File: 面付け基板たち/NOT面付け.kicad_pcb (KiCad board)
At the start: 2 copper layers, 62.9 x 53.3 mm, 45 parts, among them J1 Conn_01x01, J2 Conn_01x02, J3 Conn_01x02

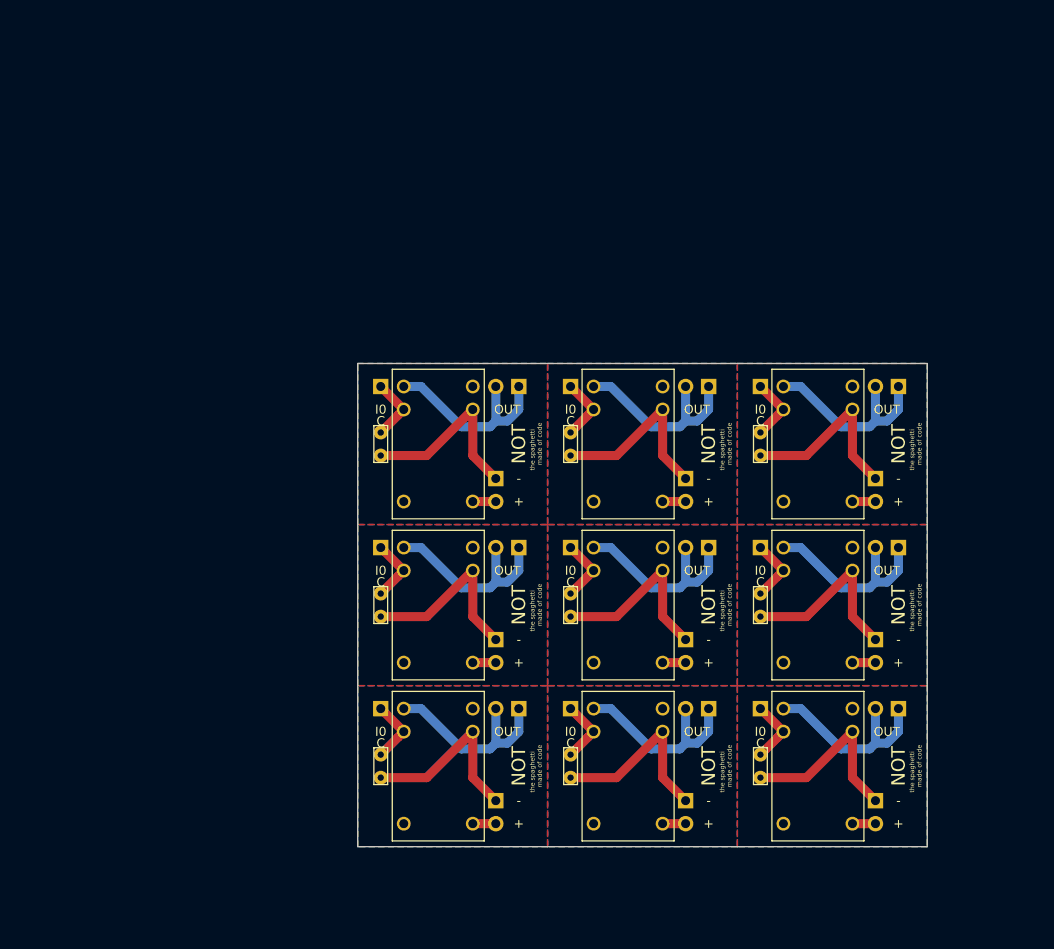
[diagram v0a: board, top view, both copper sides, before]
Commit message: Add files via upload
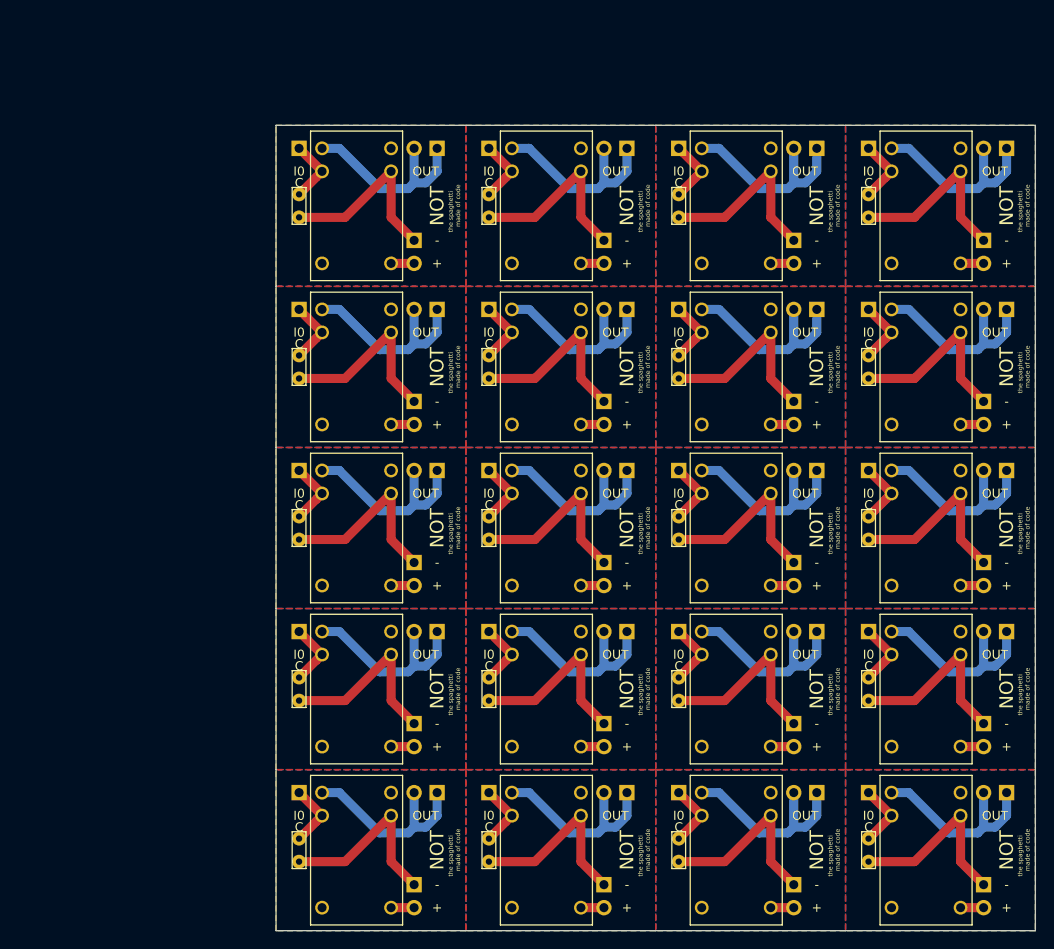
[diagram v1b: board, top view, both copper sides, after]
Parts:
- removed the C1 at (117.5, 116.2)
- removed the C1 at (96.5, 116.2)
- removed the C1 at (75.6, 116.2)
- removed the C1 at (117.5, 98.4)
- removed the C1 at (96.5, 98.4)
- removed the C1 at (75.6, 98.4)
- removed the C1 at (117.5, 80.6)
- removed the C1 at (96.5, 80.6)
- removed the J1 at (117.5, 108.6)
- removed the J1 at (96.5, 108.6)
- removed the J1 at (75.6, 108.6)
- removed the J1 at (117.5, 90.8)
- removed the J1 at (96.5, 90.8)
- removed the J1 at (75.6, 90.8)
- removed the J1 at (117.5, 73.0)
- removed the J1 at (96.5, 73.0)
- removed the J2 at (132.7, 108.6)
- removed the J2 at (111.8, 108.6)
- removed the J2 at (90.8, 108.6)
- removed the J2 at (132.7, 90.8)
- removed the J2 at (111.8, 90.8)
- removed the J2 at (90.8, 90.8)
- removed the J2 at (132.7, 73.0)
- removed the J2 at (111.8, 73.0)
- removed the J3 at (130.2, 118.7)
- removed the J3 at (109.2, 118.7)
- removed the J3 at (88.3, 118.7)
- removed the J3 at (130.2, 101.0)
- removed the J3 at (109.2, 101.0)
- removed the J3 at (88.3, 101.0)
- removed the J3 at (130.2, 83.2)
- removed the J3 at (109.2, 83.2)
- removed the SPDT1 at (125.1, 113.7)
- removed the SPDT1 at (104.1, 113.7)
- removed the SPDT1 at (83.2, 113.7)
- removed the SPDT1 at (125.1, 95.9)
- removed the SPDT1 at (104.1, 95.9)
- removed the SPDT1 at (83.2, 95.9)
- removed the SPDT1 at (125.1, 78.1)
- removed the SPDT1 at (104.1, 78.1)
- added C1: C, MiyakeFootprintLib:Condensor, F.Cu at (129.4, 125.5)
- added C1: C, MiyakeFootprintLib:Condensor, F.Cu at (108.5, 89.9)
- added C1: C, MiyakeFootprintLib:Condensor, F.Cu at (87.5, 89.9)
- added C1: C, MiyakeFootprintLib:Condensor, F.Cu at (66.5, 89.9)
- added C1: C, MiyakeFootprintLib:Condensor, F.Cu at (129.4, 72.1)
- added C1: C, MiyakeFootprintLib:Condensor, F.Cu at (108.5, 72.1)
- added C1: C, MiyakeFootprintLib:Condensor, F.Cu at (87.5, 72.1)
- added C1: C, MiyakeFootprintLib:Condensor, F.Cu at (66.5, 72.1)
- added C1: C, MiyakeFootprintLib:Condensor, F.Cu at (129.4, 54.4)
- added C1: C, MiyakeFootprintLib:Condensor, F.Cu at (108.5, 54.4)
- added C1: C, MiyakeFootprintLib:Condensor, F.Cu at (87.5, 54.4)
- added C1: C, MiyakeFootprintLib:Condensor, F.Cu at (108.5, 125.5)
- added C1: C, MiyakeFootprintLib:Condensor, F.Cu at (87.5, 125.5)
- added C1: C, MiyakeFootprintLib:Condensor, F.Cu at (66.5, 125.5)
- added C1: C, MiyakeFootprintLib:Condensor, F.Cu at (129.4, 107.7)
- added C1: C, MiyakeFootprintLib:Condensor, F.Cu at (108.5, 107.7)
- added C1: C, MiyakeFootprintLib:Condensor, F.Cu at (87.5, 107.7)
- added C1: C, MiyakeFootprintLib:Condensor, F.Cu at (66.5, 107.7)
- added C1: C, MiyakeFootprintLib:Condensor, F.Cu at (129.4, 89.9)
- added J1: Conn_01x01, Connector_PinHeader_2.54mm:PinHeader_1x01_P2.54mm_Vertical, B.Cu at (129.4, 117.9)
- added J1: Conn_01x01, Connector_PinHeader_2.54mm:PinHeader_1x01_P2.54mm_Vertical, B.Cu at (108.5, 82.3)
- added J1: Conn_01x01, Connector_PinHeader_2.54mm:PinHeader_1x01_P2.54mm_Vertical, B.Cu at (87.5, 82.3)
- added J1: Conn_01x01, Connector_PinHeader_2.54mm:PinHeader_1x01_P2.54mm_Vertical, B.Cu at (66.5, 82.3)
- added J1: Conn_01x01, Connector_PinHeader_2.54mm:PinHeader_1x01_P2.54mm_Vertical, B.Cu at (129.4, 64.5)
- added J1: Conn_01x01, Connector_PinHeader_2.54mm:PinHeader_1x01_P2.54mm_Vertical, B.Cu at (108.5, 64.5)
- added J1: Conn_01x01, Connector_PinHeader_2.54mm:PinHeader_1x01_P2.54mm_Vertical, B.Cu at (87.5, 64.5)
- added J1: Conn_01x01, Connector_PinHeader_2.54mm:PinHeader_1x01_P2.54mm_Vertical, B.Cu at (66.5, 64.5)
- added J1: Conn_01x01, Connector_PinHeader_2.54mm:PinHeader_1x01_P2.54mm_Vertical, B.Cu at (129.4, 46.7)
- added J1: Conn_01x01, Connector_PinHeader_2.54mm:PinHeader_1x01_P2.54mm_Vertical, B.Cu at (108.5, 46.7)
- added J1: Conn_01x01, Connector_PinHeader_2.54mm:PinHeader_1x01_P2.54mm_Vertical, B.Cu at (87.5, 46.7)
- added J1: Conn_01x01, Connector_PinHeader_2.54mm:PinHeader_1x01_P2.54mm_Vertical, B.Cu at (108.5, 117.9)
- added J1: Conn_01x01, Connector_PinHeader_2.54mm:PinHeader_1x01_P2.54mm_Vertical, B.Cu at (87.5, 117.9)
- added J1: Conn_01x01, Connector_PinHeader_2.54mm:PinHeader_1x01_P2.54mm_Vertical, B.Cu at (66.5, 117.9)
- added J1: Conn_01x01, Connector_PinHeader_2.54mm:PinHeader_1x01_P2.54mm_Vertical, B.Cu at (129.4, 100.1)
- added J1: Conn_01x01, Connector_PinHeader_2.54mm:PinHeader_1x01_P2.54mm_Vertical, B.Cu at (108.5, 100.1)
- added J1: Conn_01x01, Connector_PinHeader_2.54mm:PinHeader_1x01_P2.54mm_Vertical, B.Cu at (87.5, 100.1)
- added J1: Conn_01x01, Connector_PinHeader_2.54mm:PinHeader_1x01_P2.54mm_Vertical, B.Cu at (66.5, 100.1)
- added J1: Conn_01x01, Connector_PinHeader_2.54mm:PinHeader_1x01_P2.54mm_Vertical, B.Cu at (129.4, 82.3)
- added J2: Conn_01x02, Connector_PinHeader_2.54mm:PinHeader_1x02_P2.54mm_Vertical, B.Cu at (144.7, 117.9)
- added J2: Conn_01x02, Connector_PinHeader_2.54mm:PinHeader_1x02_P2.54mm_Vertical, B.Cu at (123.7, 82.3)
- added J2: Conn_01x02, Connector_PinHeader_2.54mm:PinHeader_1x02_P2.54mm_Vertical, B.Cu at (102.7, 82.3)
- added J2: Conn_01x02, Connector_PinHeader_2.54mm:PinHeader_1x02_P2.54mm_Vertical, B.Cu at (81.8, 82.3)
- added J2: Conn_01x02, Connector_PinHeader_2.54mm:PinHeader_1x02_P2.54mm_Vertical, B.Cu at (144.7, 64.5)
- added J2: Conn_01x02, Connector_PinHeader_2.54mm:PinHeader_1x02_P2.54mm_Vertical, B.Cu at (123.7, 64.5)
- added J2: Conn_01x02, Connector_PinHeader_2.54mm:PinHeader_1x02_P2.54mm_Vertical, B.Cu at (102.7, 64.5)
- added J2: Conn_01x02, Connector_PinHeader_2.54mm:PinHeader_1x02_P2.54mm_Vertical, B.Cu at (81.8, 64.5)
- added J2: Conn_01x02, Connector_PinHeader_2.54mm:PinHeader_1x02_P2.54mm_Vertical, B.Cu at (144.7, 46.7)
- added J2: Conn_01x02, Connector_PinHeader_2.54mm:PinHeader_1x02_P2.54mm_Vertical, B.Cu at (123.7, 46.7)
- added J2: Conn_01x02, Connector_PinHeader_2.54mm:PinHeader_1x02_P2.54mm_Vertical, B.Cu at (102.7, 46.7)
- added J2: Conn_01x02, Connector_PinHeader_2.54mm:PinHeader_1x02_P2.54mm_Vertical, B.Cu at (123.7, 117.9)
- added J2: Conn_01x02, Connector_PinHeader_2.54mm:PinHeader_1x02_P2.54mm_Vertical, B.Cu at (102.7, 117.9)
- added J2: Conn_01x02, Connector_PinHeader_2.54mm:PinHeader_1x02_P2.54mm_Vertical, B.Cu at (81.8, 117.9)
- added J2: Conn_01x02, Connector_PinHeader_2.54mm:PinHeader_1x02_P2.54mm_Vertical, B.Cu at (144.7, 100.1)
- added J2: Conn_01x02, Connector_PinHeader_2.54mm:PinHeader_1x02_P2.54mm_Vertical, B.Cu at (123.7, 100.1)
- added J2: Conn_01x02, Connector_PinHeader_2.54mm:PinHeader_1x02_P2.54mm_Vertical, B.Cu at (102.7, 100.1)
- added J2: Conn_01x02, Connector_PinHeader_2.54mm:PinHeader_1x02_P2.54mm_Vertical, B.Cu at (81.8, 100.1)
- added J2: Conn_01x02, Connector_PinHeader_2.54mm:PinHeader_1x02_P2.54mm_Vertical, B.Cu at (144.7, 82.3)
- added J3: Conn_01x02, Connector_PinHeader_2.54mm:PinHeader_1x02_P2.54mm_Vertical, B.Cu at (142.1, 128.0)
- added J3: Conn_01x02, Connector_PinHeader_2.54mm:PinHeader_1x02_P2.54mm_Vertical, B.Cu at (121.2, 92.5)
- added J3: Conn_01x02, Connector_PinHeader_2.54mm:PinHeader_1x02_P2.54mm_Vertical, B.Cu at (100.2, 92.5)
- added J3: Conn_01x02, Connector_PinHeader_2.54mm:PinHeader_1x02_P2.54mm_Vertical, B.Cu at (79.2, 92.5)
- added J3: Conn_01x02, Connector_PinHeader_2.54mm:PinHeader_1x02_P2.54mm_Vertical, B.Cu at (142.1, 74.7)
- added J3: Conn_01x02, Connector_PinHeader_2.54mm:PinHeader_1x02_P2.54mm_Vertical, B.Cu at (121.2, 74.7)
- added J3: Conn_01x02, Connector_PinHeader_2.54mm:PinHeader_1x02_P2.54mm_Vertical, B.Cu at (100.2, 74.7)
- added J3: Conn_01x02, Connector_PinHeader_2.54mm:PinHeader_1x02_P2.54mm_Vertical, B.Cu at (79.2, 74.7)
- added J3: Conn_01x02, Connector_PinHeader_2.54mm:PinHeader_1x02_P2.54mm_Vertical, B.Cu at (142.1, 56.9)
- added J3: Conn_01x02, Connector_PinHeader_2.54mm:PinHeader_1x02_P2.54mm_Vertical, B.Cu at (121.2, 56.9)
- added J3: Conn_01x02, Connector_PinHeader_2.54mm:PinHeader_1x02_P2.54mm_Vertical, B.Cu at (100.2, 56.9)
- added J3: Conn_01x02, Connector_PinHeader_2.54mm:PinHeader_1x02_P2.54mm_Vertical, B.Cu at (121.2, 128.0)
- added J3: Conn_01x02, Connector_PinHeader_2.54mm:PinHeader_1x02_P2.54mm_Vertical, B.Cu at (100.2, 128.0)
- added J3: Conn_01x02, Connector_PinHeader_2.54mm:PinHeader_1x02_P2.54mm_Vertical, B.Cu at (79.2, 128.0)
- added J3: Conn_01x02, Connector_PinHeader_2.54mm:PinHeader_1x02_P2.54mm_Vertical, B.Cu at (142.1, 110.2)
- added J3: Conn_01x02, Connector_PinHeader_2.54mm:PinHeader_1x02_P2.54mm_Vertical, B.Cu at (121.2, 110.2)
- added J3: Conn_01x02, Connector_PinHeader_2.54mm:PinHeader_1x02_P2.54mm_Vertical, B.Cu at (100.2, 110.2)
- added J3: Conn_01x02, Connector_PinHeader_2.54mm:PinHeader_1x02_P2.54mm_Vertical, B.Cu at (79.2, 110.2)
- added J3: Conn_01x02, Connector_PinHeader_2.54mm:PinHeader_1x02_P2.54mm_Vertical, B.Cu at (142.1, 92.5)
- added SPDT1: 946H-1C-24D, MiyakeFootprintLib:946H-1C-24D, F.Cu at (137.0, 122.9)
- added SPDT1: 946H-1C-24D, MiyakeFootprintLib:946H-1C-24D, F.Cu at (116.1, 87.4)
- added SPDT1: 946H-1C-24D, MiyakeFootprintLib:946H-1C-24D, F.Cu at (95.1, 87.4)
- added SPDT1: 946H-1C-24D, MiyakeFootprintLib:946H-1C-24D, F.Cu at (74.2, 87.4)
- added SPDT1: 946H-1C-24D, MiyakeFootprintLib:946H-1C-24D, F.Cu at (137.0, 69.6)
- added SPDT1: 946H-1C-24D, MiyakeFootprintLib:946H-1C-24D, F.Cu at (116.1, 69.6)
- added SPDT1: 946H-1C-24D, MiyakeFootprintLib:946H-1C-24D, F.Cu at (95.1, 69.6)
- added SPDT1: 946H-1C-24D, MiyakeFootprintLib:946H-1C-24D, F.Cu at (74.2, 69.6)
- added SPDT1: 946H-1C-24D, MiyakeFootprintLib:946H-1C-24D, F.Cu at (137.0, 51.8)
- added SPDT1: 946H-1C-24D, MiyakeFootprintLib:946H-1C-24D, F.Cu at (116.1, 51.8)
- added SPDT1: 946H-1C-24D, MiyakeFootprintLib:946H-1C-24D, F.Cu at (95.1, 51.8)
- added SPDT1: 946H-1C-24D, MiyakeFootprintLib:946H-1C-24D, F.Cu at (116.1, 122.9)
- added SPDT1: 946H-1C-24D, MiyakeFootprintLib:946H-1C-24D, F.Cu at (95.1, 122.9)
- added SPDT1: 946H-1C-24D, MiyakeFootprintLib:946H-1C-24D, F.Cu at (74.2, 122.9)
- added SPDT1: 946H-1C-24D, MiyakeFootprintLib:946H-1C-24D, F.Cu at (137.0, 105.2)
- added SPDT1: 946H-1C-24D, MiyakeFootprintLib:946H-1C-24D, F.Cu at (116.1, 105.2)
- added SPDT1: 946H-1C-24D, MiyakeFootprintLib:946H-1C-24D, F.Cu at (95.1, 105.2)
- added SPDT1: 946H-1C-24D, MiyakeFootprintLib:946H-1C-24D, F.Cu at (74.2, 105.2)
- added SPDT1: 946H-1C-24D, MiyakeFootprintLib:946H-1C-24D, F.Cu at (137.0, 87.4)
- moved J2 27.8 mm to (81.8, 46.7)
- moved J1 27.8 mm to (66.5, 46.7)
- moved J3 27.8 mm to (79.2, 56.9)
- moved SPDT1 27.8 mm to (74.2, 51.8)
- moved C1 27.8 mm to (66.5, 54.4)
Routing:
- net Net-(J2-Pad1): track 195.1 -> 433.6 mm
- net GND: track 188.4 -> 418.7 mm
- net Net-(C1-Pad2): track 64.7 -> 143.7 mm
- net +24V: track 22.9 -> 50.8 mm
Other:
- board size 62.9 x 53.3 mm -> 83.8 x 88.9 mm
- board text removed: "V-CUT"

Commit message: Add files via upload
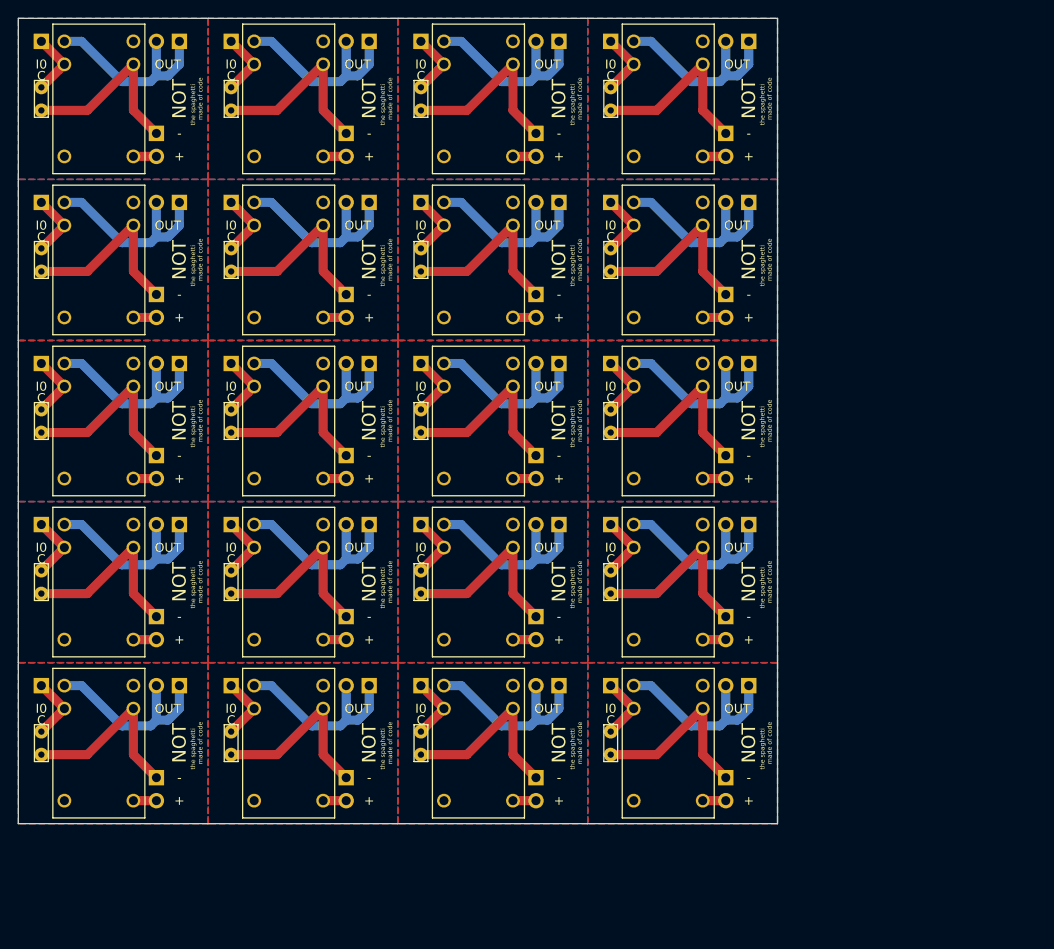
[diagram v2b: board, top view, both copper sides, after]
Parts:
- removed the C1 at (129.4, 125.5)
- removed the C1 at (108.5, 89.9)
- removed the C1 at (87.5, 89.9)
- removed the C1 at (66.5, 89.9)
- removed the C1 at (129.4, 72.1)
- removed the C1 at (108.5, 72.1)
- removed the C1 at (87.5, 72.1)
- removed the C1 at (66.5, 72.1)
- removed the C1 at (129.4, 54.4)
- removed the C1 at (108.5, 54.4)
- removed the C1 at (87.5, 54.4)
- removed the C1 at (108.5, 125.5)
- removed the C1 at (87.5, 125.5)
- removed the C1 at (66.5, 125.5)
- removed the C1 at (129.4, 107.7)
- removed the C1 at (108.5, 107.7)
- removed the C1 at (87.5, 107.7)
- removed the C1 at (66.5, 107.7)
- removed the C1 at (129.4, 89.9)
- removed the J1 at (129.4, 117.9)
- removed the J1 at (108.5, 82.3)
- removed the J1 at (87.5, 82.3)
- removed the J1 at (66.5, 82.3)
- removed the J1 at (129.4, 64.5)
- removed the J1 at (108.5, 64.5)
- removed the J1 at (87.5, 64.5)
- removed the J1 at (66.5, 64.5)
- removed the J1 at (129.4, 46.7)
- removed the J1 at (108.5, 46.7)
- removed the J1 at (87.5, 46.7)
- removed the J1 at (108.5, 117.9)
- removed the J1 at (87.5, 117.9)
- removed the J1 at (66.5, 117.9)
- removed the J1 at (129.4, 100.1)
- removed the J1 at (108.5, 100.1)
- removed the J1 at (87.5, 100.1)
- removed the J1 at (66.5, 100.1)
- removed the J1 at (129.4, 82.3)
- removed the J2 at (144.7, 117.9)
- removed the J2 at (123.7, 82.3)
- removed the J2 at (102.7, 82.3)
- removed the J2 at (81.8, 82.3)
- removed the J2 at (144.7, 64.5)
- removed the J2 at (123.7, 64.5)
- removed the J2 at (102.7, 64.5)
- removed the J2 at (81.8, 64.5)
- removed the J2 at (144.7, 46.7)
- removed the J2 at (123.7, 46.7)
- removed the J2 at (102.7, 46.7)
- removed the J2 at (123.7, 117.9)
- removed the J2 at (102.7, 117.9)
- removed the J2 at (81.8, 117.9)
- removed the J2 at (144.7, 100.1)
- removed the J2 at (123.7, 100.1)
- removed the J2 at (102.7, 100.1)
- removed the J2 at (81.8, 100.1)
- removed the J2 at (144.7, 82.3)
- removed the J3 at (142.1, 128.0)
- removed the J3 at (121.2, 92.5)
- removed the J3 at (100.2, 92.5)
- removed the J3 at (79.2, 92.5)
- removed the J3 at (142.1, 74.7)
- removed the J3 at (121.2, 74.7)
- removed the J3 at (100.2, 74.7)
- removed the J3 at (79.2, 74.7)
- removed the J3 at (142.1, 56.9)
- removed the J3 at (121.2, 56.9)
- removed the J3 at (100.2, 56.9)
- removed the J3 at (121.2, 128.0)
- removed the J3 at (100.2, 128.0)
- removed the J3 at (79.2, 128.0)
- removed the J3 at (142.1, 110.2)
- removed the J3 at (121.2, 110.2)
- removed the J3 at (100.2, 110.2)
- removed the J3 at (79.2, 110.2)
- removed the J3 at (142.1, 92.5)
- removed the SPDT1 at (137.0, 122.9)
- removed the SPDT1 at (116.1, 87.4)
- removed the SPDT1 at (95.1, 87.4)
- removed the SPDT1 at (74.2, 87.4)
- removed the SPDT1 at (137.0, 69.6)
- removed the SPDT1 at (116.1, 69.6)
- removed the SPDT1 at (95.1, 69.6)
- removed the SPDT1 at (74.2, 69.6)
- removed the SPDT1 at (137.0, 51.8)
- removed the SPDT1 at (116.1, 51.8)
- removed the SPDT1 at (95.1, 51.8)
- removed the SPDT1 at (116.1, 122.9)
- removed the SPDT1 at (95.1, 122.9)
- removed the SPDT1 at (74.2, 122.9)
- removed the SPDT1 at (137.0, 105.2)
- removed the SPDT1 at (116.1, 105.2)
- removed the SPDT1 at (95.1, 105.2)
- removed the SPDT1 at (74.2, 105.2)
- removed the SPDT1 at (137.0, 87.4)
- added C1: C, MiyakeFootprintLib:Condensor, F.Cu at (101.0, 113.7)
- added C1: C, MiyakeFootprintLib:Condensor, F.Cu at (80.0, 78.1)
- added C1: C, MiyakeFootprintLib:Condensor, F.Cu at (59.0, 78.1)
- added C1: C, MiyakeFootprintLib:Condensor, F.Cu at (38.1, 78.1)
- added C1: C, MiyakeFootprintLib:Condensor, F.Cu at (101.0, 60.3)
- added C1: C, MiyakeFootprintLib:Condensor, F.Cu at (80.0, 60.3)
- added C1: C, MiyakeFootprintLib:Condensor, F.Cu at (59.0, 60.3)
- added C1: C, MiyakeFootprintLib:Condensor, F.Cu at (38.1, 60.3)
- added C1: C, MiyakeFootprintLib:Condensor, F.Cu at (101.0, 42.5)
- added C1: C, MiyakeFootprintLib:Condensor, F.Cu at (80.0, 42.5)
- added C1: C, MiyakeFootprintLib:Condensor, F.Cu at (59.0, 42.5)
- added C1: C, MiyakeFootprintLib:Condensor, F.Cu at (80.0, 113.7)
- added C1: C, MiyakeFootprintLib:Condensor, F.Cu at (59.0, 113.7)
- added C1: C, MiyakeFootprintLib:Condensor, F.Cu at (38.1, 113.7)
- added C1: C, MiyakeFootprintLib:Condensor, F.Cu at (101.0, 95.9)
- added C1: C, MiyakeFootprintLib:Condensor, F.Cu at (80.0, 95.9)
- added C1: C, MiyakeFootprintLib:Condensor, F.Cu at (59.0, 95.9)
- added C1: C, MiyakeFootprintLib:Condensor, F.Cu at (38.1, 95.9)
- added C1: C, MiyakeFootprintLib:Condensor, F.Cu at (101.0, 78.1)
- added J1: Conn_01x01, Connector_PinHeader_2.54mm:PinHeader_1x01_P2.54mm_Vertical, B.Cu at (101.0, 106.0)
- added J1: Conn_01x01, Connector_PinHeader_2.54mm:PinHeader_1x01_P2.54mm_Vertical, B.Cu at (80.0, 70.5)
- added J1: Conn_01x01, Connector_PinHeader_2.54mm:PinHeader_1x01_P2.54mm_Vertical, B.Cu at (59.0, 70.5)
- added J1: Conn_01x01, Connector_PinHeader_2.54mm:PinHeader_1x01_P2.54mm_Vertical, B.Cu at (38.1, 70.5)
- added J1: Conn_01x01, Connector_PinHeader_2.54mm:PinHeader_1x01_P2.54mm_Vertical, B.Cu at (101.0, 52.7)
- added J1: Conn_01x01, Connector_PinHeader_2.54mm:PinHeader_1x01_P2.54mm_Vertical, B.Cu at (80.0, 52.7)
- added J1: Conn_01x01, Connector_PinHeader_2.54mm:PinHeader_1x01_P2.54mm_Vertical, B.Cu at (59.0, 52.7)
- added J1: Conn_01x01, Connector_PinHeader_2.54mm:PinHeader_1x01_P2.54mm_Vertical, B.Cu at (38.1, 52.7)
- added J1: Conn_01x01, Connector_PinHeader_2.54mm:PinHeader_1x01_P2.54mm_Vertical, B.Cu at (101.0, 34.9)
- added J1: Conn_01x01, Connector_PinHeader_2.54mm:PinHeader_1x01_P2.54mm_Vertical, B.Cu at (80.0, 34.9)
- added J1: Conn_01x01, Connector_PinHeader_2.54mm:PinHeader_1x01_P2.54mm_Vertical, B.Cu at (59.0, 34.9)
- added J1: Conn_01x01, Connector_PinHeader_2.54mm:PinHeader_1x01_P2.54mm_Vertical, B.Cu at (80.0, 106.0)
- added J1: Conn_01x01, Connector_PinHeader_2.54mm:PinHeader_1x01_P2.54mm_Vertical, B.Cu at (59.0, 106.0)
- added J1: Conn_01x01, Connector_PinHeader_2.54mm:PinHeader_1x01_P2.54mm_Vertical, B.Cu at (38.1, 106.0)
- added J1: Conn_01x01, Connector_PinHeader_2.54mm:PinHeader_1x01_P2.54mm_Vertical, B.Cu at (101.0, 88.3)
- added J1: Conn_01x01, Connector_PinHeader_2.54mm:PinHeader_1x01_P2.54mm_Vertical, B.Cu at (80.0, 88.3)
- added J1: Conn_01x01, Connector_PinHeader_2.54mm:PinHeader_1x01_P2.54mm_Vertical, B.Cu at (59.0, 88.3)
- added J1: Conn_01x01, Connector_PinHeader_2.54mm:PinHeader_1x01_P2.54mm_Vertical, B.Cu at (38.1, 88.3)
- added J1: Conn_01x01, Connector_PinHeader_2.54mm:PinHeader_1x01_P2.54mm_Vertical, B.Cu at (101.0, 70.5)
- added J2: Conn_01x02, Connector_PinHeader_2.54mm:PinHeader_1x02_P2.54mm_Vertical, B.Cu at (116.2, 106.0)
- added J2: Conn_01x02, Connector_PinHeader_2.54mm:PinHeader_1x02_P2.54mm_Vertical, B.Cu at (95.2, 70.5)
- added J2: Conn_01x02, Connector_PinHeader_2.54mm:PinHeader_1x02_P2.54mm_Vertical, B.Cu at (74.3, 70.5)
- added J2: Conn_01x02, Connector_PinHeader_2.54mm:PinHeader_1x02_P2.54mm_Vertical, B.Cu at (53.3, 70.5)
- added J2: Conn_01x02, Connector_PinHeader_2.54mm:PinHeader_1x02_P2.54mm_Vertical, B.Cu at (116.2, 52.7)
- added J2: Conn_01x02, Connector_PinHeader_2.54mm:PinHeader_1x02_P2.54mm_Vertical, B.Cu at (95.2, 52.7)
- added J2: Conn_01x02, Connector_PinHeader_2.54mm:PinHeader_1x02_P2.54mm_Vertical, B.Cu at (74.3, 52.7)
- added J2: Conn_01x02, Connector_PinHeader_2.54mm:PinHeader_1x02_P2.54mm_Vertical, B.Cu at (53.3, 52.7)
- added J2: Conn_01x02, Connector_PinHeader_2.54mm:PinHeader_1x02_P2.54mm_Vertical, B.Cu at (116.2, 34.9)
- added J2: Conn_01x02, Connector_PinHeader_2.54mm:PinHeader_1x02_P2.54mm_Vertical, B.Cu at (95.2, 34.9)
- added J2: Conn_01x02, Connector_PinHeader_2.54mm:PinHeader_1x02_P2.54mm_Vertical, B.Cu at (74.3, 34.9)
- added J2: Conn_01x02, Connector_PinHeader_2.54mm:PinHeader_1x02_P2.54mm_Vertical, B.Cu at (95.2, 106.0)
- added J2: Conn_01x02, Connector_PinHeader_2.54mm:PinHeader_1x02_P2.54mm_Vertical, B.Cu at (74.3, 106.0)
- added J2: Conn_01x02, Connector_PinHeader_2.54mm:PinHeader_1x02_P2.54mm_Vertical, B.Cu at (53.3, 106.0)
- added J2: Conn_01x02, Connector_PinHeader_2.54mm:PinHeader_1x02_P2.54mm_Vertical, B.Cu at (116.2, 88.3)
- added J2: Conn_01x02, Connector_PinHeader_2.54mm:PinHeader_1x02_P2.54mm_Vertical, B.Cu at (95.2, 88.3)
- added J2: Conn_01x02, Connector_PinHeader_2.54mm:PinHeader_1x02_P2.54mm_Vertical, B.Cu at (74.3, 88.3)
- added J2: Conn_01x02, Connector_PinHeader_2.54mm:PinHeader_1x02_P2.54mm_Vertical, B.Cu at (53.3, 88.3)
- added J2: Conn_01x02, Connector_PinHeader_2.54mm:PinHeader_1x02_P2.54mm_Vertical, B.Cu at (116.2, 70.5)
- added J3: Conn_01x02, Connector_PinHeader_2.54mm:PinHeader_1x02_P2.54mm_Vertical, B.Cu at (113.7, 116.2)
- added J3: Conn_01x02, Connector_PinHeader_2.54mm:PinHeader_1x02_P2.54mm_Vertical, B.Cu at (92.7, 80.6)
- added J3: Conn_01x02, Connector_PinHeader_2.54mm:PinHeader_1x02_P2.54mm_Vertical, B.Cu at (71.8, 80.6)
- added J3: Conn_01x02, Connector_PinHeader_2.54mm:PinHeader_1x02_P2.54mm_Vertical, B.Cu at (50.8, 80.6)
- added J3: Conn_01x02, Connector_PinHeader_2.54mm:PinHeader_1x02_P2.54mm_Vertical, B.Cu at (113.7, 62.9)
- added J3: Conn_01x02, Connector_PinHeader_2.54mm:PinHeader_1x02_P2.54mm_Vertical, B.Cu at (92.7, 62.9)
- added J3: Conn_01x02, Connector_PinHeader_2.54mm:PinHeader_1x02_P2.54mm_Vertical, B.Cu at (71.8, 62.9)
- added J3: Conn_01x02, Connector_PinHeader_2.54mm:PinHeader_1x02_P2.54mm_Vertical, B.Cu at (50.8, 62.9)
- added J3: Conn_01x02, Connector_PinHeader_2.54mm:PinHeader_1x02_P2.54mm_Vertical, B.Cu at (113.7, 45.1)
- added J3: Conn_01x02, Connector_PinHeader_2.54mm:PinHeader_1x02_P2.54mm_Vertical, B.Cu at (92.7, 45.1)
- added J3: Conn_01x02, Connector_PinHeader_2.54mm:PinHeader_1x02_P2.54mm_Vertical, B.Cu at (71.8, 45.1)
- added J3: Conn_01x02, Connector_PinHeader_2.54mm:PinHeader_1x02_P2.54mm_Vertical, B.Cu at (92.7, 116.2)
- added J3: Conn_01x02, Connector_PinHeader_2.54mm:PinHeader_1x02_P2.54mm_Vertical, B.Cu at (71.8, 116.2)
- added J3: Conn_01x02, Connector_PinHeader_2.54mm:PinHeader_1x02_P2.54mm_Vertical, B.Cu at (50.8, 116.2)
- added J3: Conn_01x02, Connector_PinHeader_2.54mm:PinHeader_1x02_P2.54mm_Vertical, B.Cu at (113.7, 98.4)
- added J3: Conn_01x02, Connector_PinHeader_2.54mm:PinHeader_1x02_P2.54mm_Vertical, B.Cu at (92.7, 98.4)
- added J3: Conn_01x02, Connector_PinHeader_2.54mm:PinHeader_1x02_P2.54mm_Vertical, B.Cu at (71.8, 98.4)
- added J3: Conn_01x02, Connector_PinHeader_2.54mm:PinHeader_1x02_P2.54mm_Vertical, B.Cu at (50.8, 98.4)
- added J3: Conn_01x02, Connector_PinHeader_2.54mm:PinHeader_1x02_P2.54mm_Vertical, B.Cu at (113.7, 80.6)
- added SPDT1: 946H-1C-24D, MiyakeFootprintLib:946H-1C-24D, F.Cu at (108.6, 111.1)
- added SPDT1: 946H-1C-24D, MiyakeFootprintLib:946H-1C-24D, F.Cu at (87.6, 75.6)
- added SPDT1: 946H-1C-24D, MiyakeFootprintLib:946H-1C-24D, F.Cu at (66.7, 75.6)
- added SPDT1: 946H-1C-24D, MiyakeFootprintLib:946H-1C-24D, F.Cu at (45.7, 75.6)
- added SPDT1: 946H-1C-24D, MiyakeFootprintLib:946H-1C-24D, F.Cu at (108.6, 57.8)
- added SPDT1: 946H-1C-24D, MiyakeFootprintLib:946H-1C-24D, F.Cu at (87.6, 57.8)
- added SPDT1: 946H-1C-24D, MiyakeFootprintLib:946H-1C-24D, F.Cu at (66.7, 57.8)
- added SPDT1: 946H-1C-24D, MiyakeFootprintLib:946H-1C-24D, F.Cu at (45.7, 57.8)
- added SPDT1: 946H-1C-24D, MiyakeFootprintLib:946H-1C-24D, F.Cu at (108.6, 40.0)
- added SPDT1: 946H-1C-24D, MiyakeFootprintLib:946H-1C-24D, F.Cu at (87.6, 40.0)
- added SPDT1: 946H-1C-24D, MiyakeFootprintLib:946H-1C-24D, F.Cu at (66.7, 40.0)
- added SPDT1: 946H-1C-24D, MiyakeFootprintLib:946H-1C-24D, F.Cu at (87.6, 111.1)
- added SPDT1: 946H-1C-24D, MiyakeFootprintLib:946H-1C-24D, F.Cu at (66.7, 111.1)
- added SPDT1: 946H-1C-24D, MiyakeFootprintLib:946H-1C-24D, F.Cu at (45.7, 111.1)
- added SPDT1: 946H-1C-24D, MiyakeFootprintLib:946H-1C-24D, F.Cu at (108.6, 93.3)
- added SPDT1: 946H-1C-24D, MiyakeFootprintLib:946H-1C-24D, F.Cu at (87.6, 93.3)
- added SPDT1: 946H-1C-24D, MiyakeFootprintLib:946H-1C-24D, F.Cu at (66.7, 93.3)
- added SPDT1: 946H-1C-24D, MiyakeFootprintLib:946H-1C-24D, F.Cu at (45.7, 93.3)
- added SPDT1: 946H-1C-24D, MiyakeFootprintLib:946H-1C-24D, F.Cu at (108.6, 75.6)
- moved J3 30.8 mm to (50.8, 45.1)
- moved SPDT1 30.8 mm to (45.7, 40.0)
- moved C1 30.8 mm to (38.1, 42.5)
- moved J1 30.8 mm to (38.1, 34.9)
- moved J2 30.8 mm to (53.3, 34.9)
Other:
- outline, holes or cut-outs redrawn
- board text added: "V-CUT"
